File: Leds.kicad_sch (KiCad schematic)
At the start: 14 parts, among them SW4 SW_SPDT, SW7 SW_Push

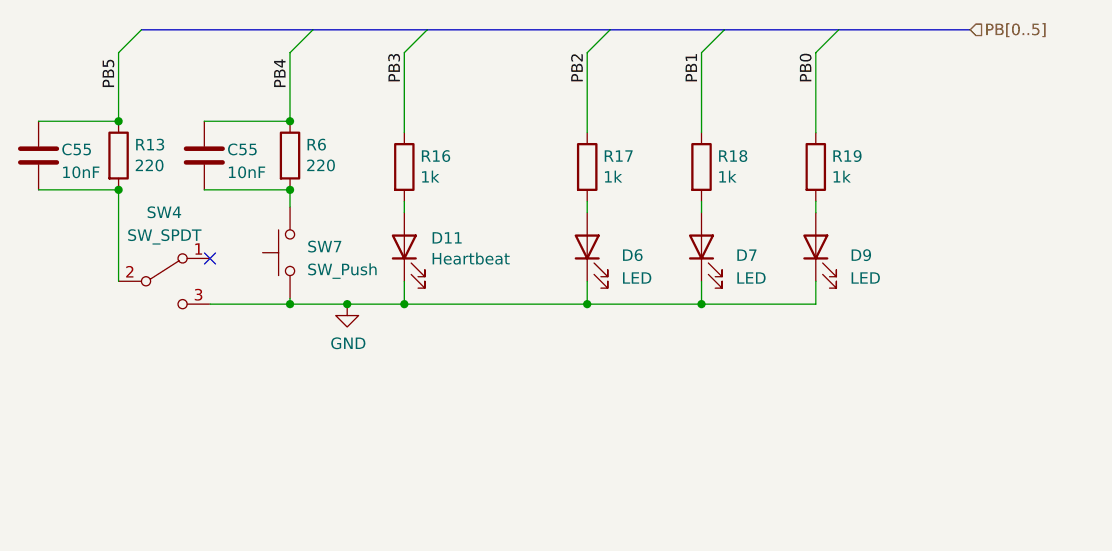
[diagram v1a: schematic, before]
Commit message: changed pins around to make routing easier
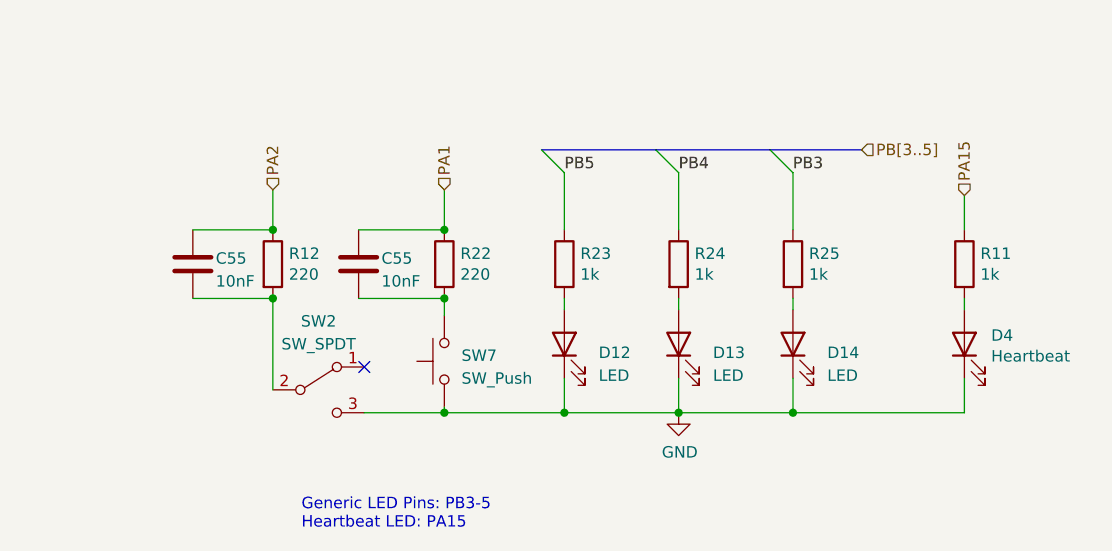
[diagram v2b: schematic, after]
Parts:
- removed C55 (x2): 10nF, Capacitor_SMD:C_0805_2012Metric, symbol Device:C
- removed D11: Heartbeat, LED_SMD:LED_0805_2012Metric, symbol Device:LED
- removed D6, D7, D9: LED, LED_SMD:LED_0805_2012Metric, symbol Device:LED
- removed R13, R6: 220, Resistor_SMD:R_0805_2012Metric, symbol Device:R
- removed R16, R17, R18, R19: 1k, Resistor_SMD:R_0805_2012Metric, symbol Device:R
- removed SW4: SW_SPDT, UTSVT_Mechanical:CJS-1200B_NDC, symbol Switch:SW_SPDT
- added C55 (x2): 10nF, Capacitor_SMD:C_0805_2012Metric, symbol Device:C
- added D12, D13, D14: LED, LED_SMD:LED_0805_2012Metric, symbol Device:LED
- added D4: Heartbeat, LED_SMD:LED_0805_2012Metric, symbol Device:LED
- added R11, R23, R24, R25: 1k, Resistor_SMD:R_0805_2012Metric, symbol Device:R
- added R12, R22: 220, Resistor_SMD:R_0805_2012Metric, symbol Device:R
- added SW2: SW_SPDT, UTSVT_Mechanical:CJS-1200B_NDC, symbol Switch:SW_SPDT
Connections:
- net GND: now also D12.1 (K), D13.1 (K), D14.1 (K), D4.1 (K), SW2.3 (C)
- net PB3: now also R25.1
- net PB4: now also R24.1
- net PB5: now also R23.1
- net at SW7.2: now also C55.2, R22.2
- new net: D4.2 (A), R11.2
- new net: D13.2 (A), R24.2
- new net: D12.2 (A), R23.2
- new net: C55.2, R12.2, SW2.2 (B)
- new net: D14.2 (A), R25.2
- new net PA1: C55.1, R22.1
- new net PA15: R11.1
- new net PA2: C55.1, R12.1
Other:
- note added: "Generic LED Pins: PB3-5 Heartbeat LED: PA15"

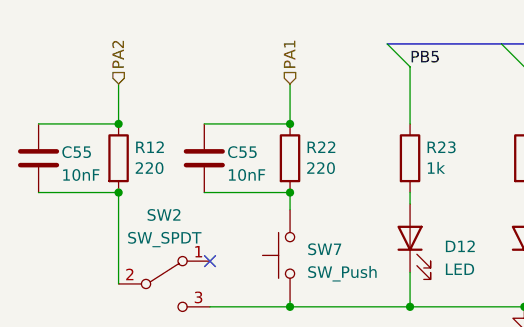
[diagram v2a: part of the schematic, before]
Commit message: Prelim layout v2 final draft (ahhhhhhhhh), also connected GPIO to STDBY and SILENT pins
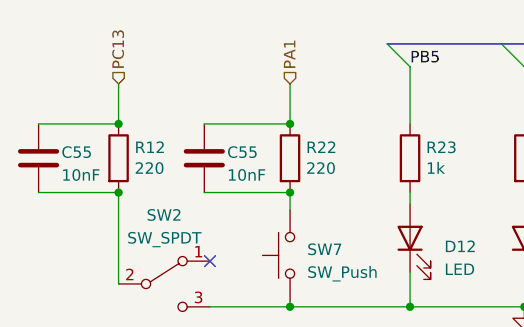
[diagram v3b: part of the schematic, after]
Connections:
- net PA2 renamed PC13
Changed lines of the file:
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@@
     (effects (font (size 1.27 1.27)) (justify left))
   )
-  (hierarchical_label "PA2" (shape input) (at 86.995 99.06 90) (fields_autoplaced)
+  (hierarchical_label "PC13" (shape input) (at 86.995 99.06 90) (fields_autoplaced)
     (effects (font (size 1.27 1.27)) (justify left))
   )

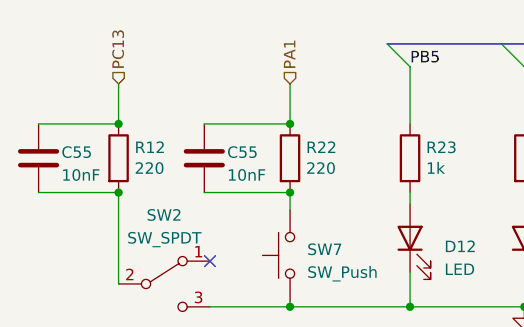
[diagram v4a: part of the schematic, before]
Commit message: added Tianda's suggestions
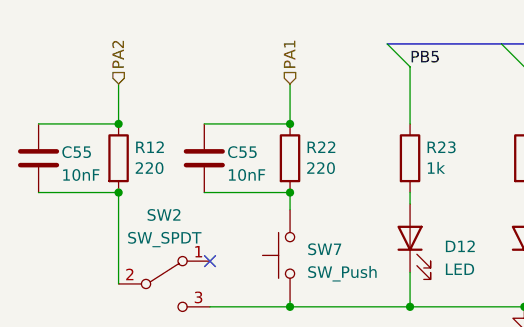
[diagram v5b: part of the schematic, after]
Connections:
- net PC13 renamed PA2
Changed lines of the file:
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@@
     (effects (font (size 1.27 1.27)) (justify left))
   )
-  (hierarchical_label "PC13" (shape input) (at 86.995 99.06 90) (fields_autoplaced)
+  (hierarchical_label "PA2" (shape input) (at 86.995 99.06 90) (fields_autoplaced)
     (effects (font (size 1.27 1.27)) (justify left))
   )
